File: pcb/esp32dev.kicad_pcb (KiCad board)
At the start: 4 copper layers, 47.6 x 20.3 mm, 26 parts, among them J3 USB-C, U1 ESP32-C3, U2 AP1117-33, U3 W25Q128JVS

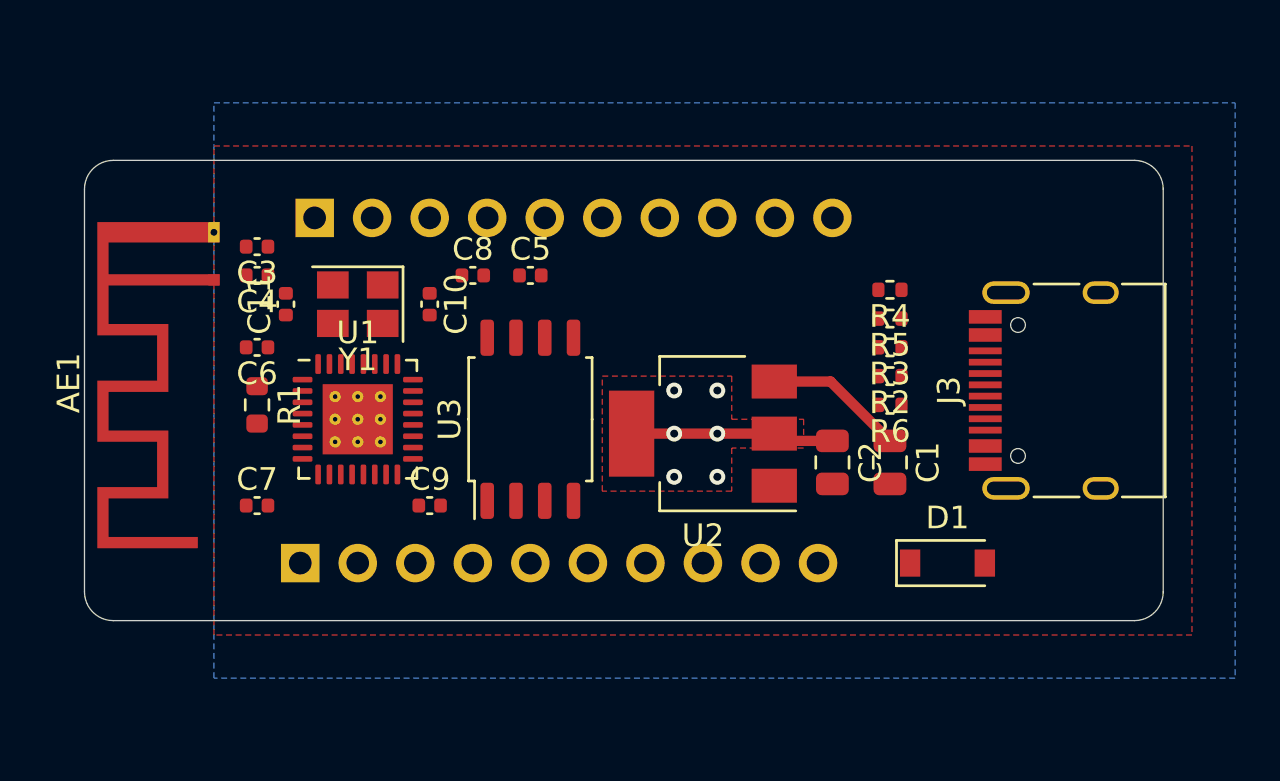
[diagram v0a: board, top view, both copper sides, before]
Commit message: Hmmm
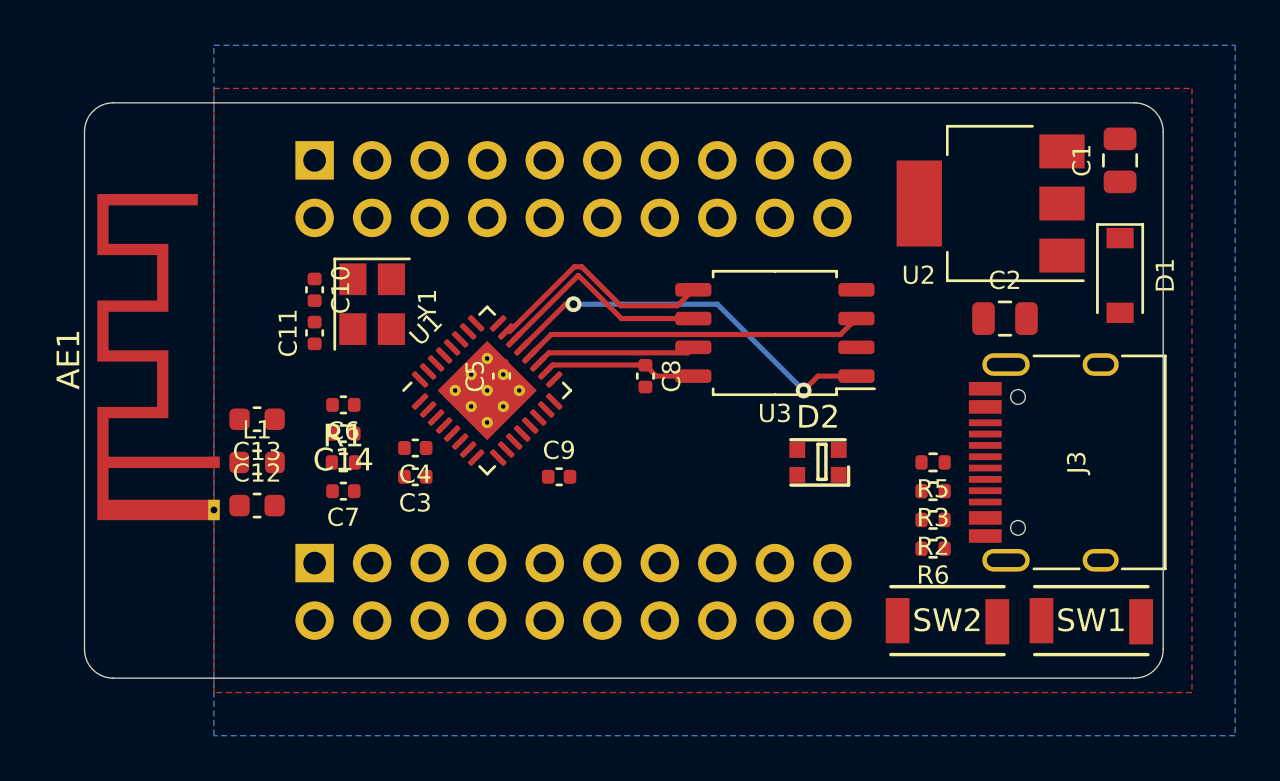
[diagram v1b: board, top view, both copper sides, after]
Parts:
- removed R4: 1.5k, Resistor_SMD:R_0402_1005Metric
- added C12: NM, Capacitor_SMD:C_0603_1608Metric, F.Cu at (109.2, 97.8)
- added C13: NM, Capacitor_SMD:C_0603_1608Metric, F.Cu at (109.2, 94.0)
- added C14: 100nF, Capacitor_SMD:C_0402_1005Metric, F.Cu at (113.0, 94.6)
- added D2: WS2812C-2020, esp32dev:LED_WS2812C-2020, F.Cu at (134.0, 95.9)
- added L1: L, Inductor_SMD:L_0603_1608Metric, F.Cu at (109.2, 95.9)
- added SW1: ~, esp32dev:TS-1088R-02526, F.Cu at (146.1, 102.9)
- added SW2: ~, esp32dev:TS-1088R-02526, F.Cu at (139.7, 102.9)
- AE1: footprint esp32dev:Texas_SWRA117D_2.4GHz_Left -> esp32dev:Texas_SWRA117D_2.4GHz_Right
- J1, J2: footprint Connector_PinHeader_2.54mm:PinHeader_1x10_P2.54mm_Vertical -> Connector_PinHeader_2.54mm:PinHeader_2x10_P2.54mm_Vertical
- R1: footprint Resistor_SMD:R_0603_1608Metric -> Resistor_SMD:R_0402_1005Metric
- Y1: value ~ -> 40MHz
- moved C1 16.8 mm to (147.3, 82.5), turned to 90 degrees
- moved U2 16.3 mm to (141.6, 84.5)
- moved D1 14.8 mm to (147.3, 87.6), turned to 270 degrees
- moved C3 12.3 mm to (116.2, 96.5)
- moved U3 11.4 mm to (132.1, 90.2), turned to 180 degrees
- moved C4 10.3 mm to (116.2, 95.2)
- moved C2 9.92 mm to (142.2, 89.5), turned to 0 degrees
- moved C8 8.82 mm to (126.4, 92.1), turned to 270 degrees
- moved AE1 8.06 mm to (107.3, 95.9)
- moved R5 6.63 mm to (139.1, 95.9)
- moved R2 6.63 mm to (139.1, 98.4)
- moved R3 6.63 mm to (139.1, 97.2)
- moved R6 6.63 mm to (139.1, 99.7)
- moved C9 5.85 mm to (122.6, 96.5)
- moved U1 5.85 mm to (119.4, 92.7), turned to 45 degrees
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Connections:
- net F_RST renamed IO12_F_RST
- net F_WP renamed IO13_F_WP
- net Net-(U1-Pad10) renamed IO5_MTDI
- net Net-(U1-Pad12) renamed IO6_MTCK
- net Net-(U1-Pad13) renamed IO7_MTDO
- net Net-(U1-Pad14) renamed IO8
- net Net-(U1-Pad15) renamed IO9
- net Net-(U1-Pad16) renamed IO10
- net Net-(U1-Pad4) renamed IO0
- net Net-(U1-Pad5) renamed IO1
- net Net-(U1-Pad6) renamed IO2
- net Net-(U1-Pad8) renamed IO3
- net Net-(U1-Pad9) renamed IO4_MTMS
- J1 pad 2: Net-(J1-Pad2) -> Net-(J1-Pad1)
- J1 pad 4: Net-(J1-Pad4) -> Net-(J1-Pad3)
- J1 pad 6: Net-(J1-Pad6) -> Net-(J1-Pad5)
- J1 pad 8: Net-(J1-Pad8) -> Net-(J1-Pad7)
- J1 pad 9: Net-(J1-Pad9) -> Net-(J1-Pad10)
- J2 pad 2: Net-(J2-Pad2) -> Net-(J2-Pad1)
- J2 pad 4: Net-(J2-Pad4) -> Net-(J2-Pad3)
- J2 pad 6: Net-(J2-Pad6) -> Net-(J2-Pad5)
- J2 pad 8: Net-(J2-Pad8) -> Net-(J2-Pad7)
- J2 pad 9: Net-(J2-Pad9) -> Net-(J2-Pad10)
- R2 pad 2: DM -> IO18_DM
- R3 pad 2: DP -> IO19_DP
- U1 pad 1: Net-(AE1-Pad1) -> Net-(C13-Pad1)
- U1 pad 25: DM -> IO18_DM
- U1 pad 26: DP -> IO19_DP
- U1 pad 27: Net-(U1-Pad27) -> IO20_U0RX
- U1 pad 28: Net-(U1-Pad28) -> IO21_U0TX
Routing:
- net F_CS: track 0.00 -> 17.4 mm, vias 0 -> 2
- net IO13_F_WP: track 0.00 -> 15.1 mm
- net F_DI: track 0.00 -> 10.4 mm
- net F_CK: track 0.00 -> 9.87 mm
- net +3V3: track 9.00 -> 0.00 mm, vias 6 -> 0
- net IO12_F_RST: track 0.00 -> 7.14 mm
- net VDD_SPI: track 0.00 -> 6.81 mm
- net VBUS: track 6.19 -> 0.00 mm
- net Net-(J2-Pad7): track 0.00 -> 2.54 mm
- net Net-(J2-Pad5): track 0.00 -> 2.54 mm
- net Net-(J2-Pad3): track 0.00 -> 2.54 mm
- net Net-(J2-Pad19): track 0.00 -> 2.54 mm
- net Net-(J2-Pad17): track 0.00 -> 2.54 mm
- net Net-(J2-Pad15): track 0.00 -> 2.54 mm
- net Net-(J2-Pad10): track 0.00 -> 2.54 mm
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- removed copper zone on F.Cu, net +3V3
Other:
- board size 47.6 x 20.3 mm -> 47.6 x 25.4 mm
